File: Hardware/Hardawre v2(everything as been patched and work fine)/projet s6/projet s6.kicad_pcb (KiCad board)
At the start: 4 copper layers, 26.4 x 19 mm, 55 parts, among them IC1 QMC5883L, J1 USB_C_Receptacle_USB2.0_14P, J2 OLED, Q1 2N7002K, SW1 Boutton 1, SW2 Boutton 2, SW5 RSTBTN, SW6 Int, SW7 boot, U1 STM32L432KCUx, U2 LTC4065AEDC, U3 LDLN022PU33R, U4 USBLC6-2SC6

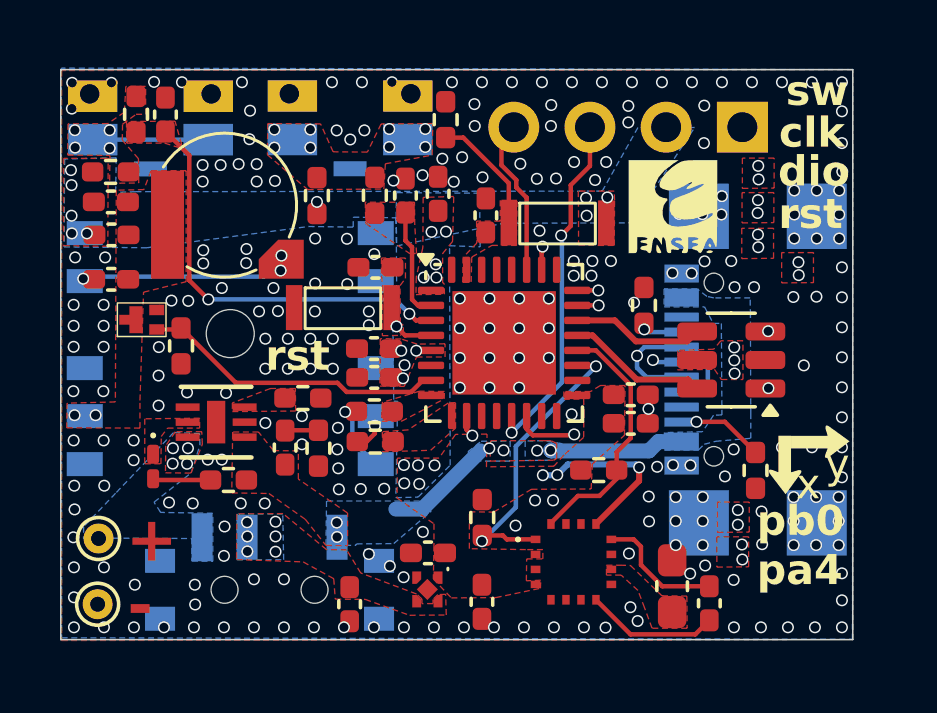
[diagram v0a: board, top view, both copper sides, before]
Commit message: gr
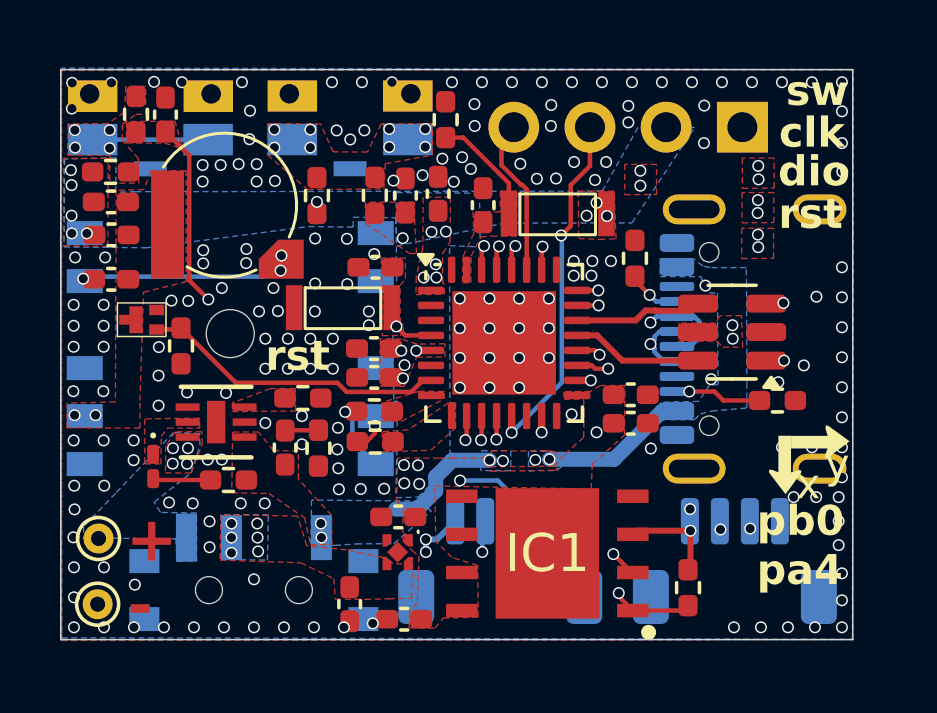
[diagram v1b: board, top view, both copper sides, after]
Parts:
- removed C11: 0.22u, Capacitor_SMD:C_0402_1005Metric_Pad0.74x0.62mm_HandSolder
- removed C12: 0.1u, Capacitor_SMD:C_0402_1005Metric_Pad0.74x0.62mm_HandSolder
- removed the G*** at (201.8, 69.6)
- removed R9: 2.2k, Resistor_SMD:R_0402_1005Metric_Pad0.72x0.64mm_HandSolder
- added J3: i2c, Connector_JST:JST_SH_BM04B-SRSS-TB_1x04-1MP_P1.00mm_Vertical, B.Cu at (203.8, 81.4)
- added J4: usart, Connector_JST:JST_SH_BM04B-SRSS-TB_1x04-1MP_P1.00mm_Vertical, B.Cu at (196.0, 81.4)
- BT1: footprint MS414:MS421R-IV03E -> MS421R-IV03E:MS421R-IV03E
- C13: value 4.7u -> 100n; footprint Capacitor_SMD:C_0603_1608Metric_Pad1.08x0.95mm_HandSolder -> Capacitor_SMD:C_0402_1005Metric_Pad0.74x0.62mm_HandSolder
- IC1: value QMC5883L -> W25Q128JVPIQ_TR; footprint QMC5883L:QMC5883L -> winbond:SON127P600X500X80-9N-D
- J1: footprint USB4110_USBC_SMT:USB4110_USBC_SMT -> USBC-WURTH:USBC-WURTH
- R8: value 2.2k -> 10k
- SW1, SW2: footprint SW_PTS840:SW_PTS840 -> PTS840:SW_PTS840
- SW5, SW7: footprint SW_KXT3:SW_KXT3 -> KXT3:SW_KXT3
- SW6: footprint SW_PCM:SW_PCM -> PCM:SW_PCM
- moved C13 9.00 mm to (192.8, 83.4), turned to 180 degrees
- moved J1 5.55 mm to (205.6, 74.0)
- moved R8 4.92 mm to (202.3, 82.3), turned to 90 degrees
- moved R4 2.44 mm to (205.2, 76.1), turned to 0 degrees
- moved R5 1.60 mm to (200.5, 71.3)
- moved U3 1.59 mm to (192.1, 80.5)
- moved C15 1.56 mm to (192.6, 80.0)
- moved U4 0.93 mm to (203.7, 73.8)
- moved IC1 0.91 mm to (197.6, 81.2), turned to 180 degrees
- moved SW6 0.52 mm to (191.9, 83.8)
- moved C18 0.35 mm to (195.4, 69.6)
- moved SW7 0.31 mm to (196.0, 70.6)
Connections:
- C13 pad 1: Net-(IC1-C1) -> +3.3V
- IC1 pad 1: COMPASSCL -> SPI_CS
- IC1 pad 2: +3.3V -> SPI_MISO
- IC1 pad 3: unconnected-(IC1-NC_1-Pad3) -> +3.3V
- IC1 pad 4: +3.3V -> GND
- IC1 pad 5: unconnected-(IC1-NC_2-Pad5) -> SPI_MOSi
- IC1 pad 6: unconnected-(IC1-NC_3-Pad6) -> SPI_SCK
- IC1 pad 7: unconnected-(IC1-NC_4-Pad7) -> +3.3V
- IC1 pad 8: Net-(IC1-STEP) -> +3.3V
- R8 pad 1: +3.3V -> SPI_CS
- R8 pad 2: COMPASSDA -> +3.3V
- U1 pad 10: unconnected-(U1-PA4-Pad10) -> SPI_CS
- U1 pad 11: unconnected-(U1-PA5-Pad11) -> SPI_SCK
- U1 pad 12: unconnected-(U1-PA6-Pad12) -> SPI_MISO
- U1 pad 15: unconnected-(U1-PB1-Pad15) -> B2
- U1 pad 18: unconnected-(U1-PA8-Pad18) -> B1
- U1 pad 2: B1 -> OSC32_IN
- U1 pad 28: unconnected-(U1-PB5-Pad28) -> SPI_MOSi
- U1 pad 29: unconnected-(U1-PB6-Pad29) -> USART_TX
- U1 pad 3: B2 -> OSC32_OUT
- U1 pad 30: unconnected-(U1-PB7-Pad30) -> USART_RX
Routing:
- net USART_RX: track 0.00 -> 13.4 mm, vias 0 -> 2
- net unconnected-(U1-PA4-Pad10): track 13.1 -> 0.00 mm, vias 3 -> 0
- net USART_TX: track 0.00 -> 12.8 mm, vias 0 -> 2
- net unconnected-(U1-PB0-Pad14): track 9.11 -> 0.00 mm, vias 3 -> 0
- net SPI_MISO: track 0.00 -> 7.17 mm, vias 0 -> 2
- net B1: track 3.70 -> 9.82 mm, vias 0 -> 2
- net B2: track 13.9 -> 19.2 mm
- net Net-(IC1-STEP): track 4.45 -> 0.00 mm
- net Net-(U1-NRST): track 18.3 -> 13.9 mm
- net Net-(IC1-SETC): track 4.27 -> 0.00 mm
- net +3.3V: track 6.27 -> 10.2 mm, vias 26 -> 27
- net SPI_CS: track 0.00 -> 3.50 mm, vias 0 -> 2
- net COMPASSDA: track 8.41 -> 9.89 mm, vias 0 -> 2
- net SWCLK: track 7.52 -> 8.70 mm
- net COMPASSCL: track 10.1 -> 8.99 mm
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- removed copper zone on F.Cu, net Net-(IC1-C1)
- removed copper zone on F.Cu, net unconnected-(U1-PA4-Pad10)
- removed copper zone on F.Cu, net unconnected-(U1-PB0-Pad14)
